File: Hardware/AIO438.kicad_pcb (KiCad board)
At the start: 2 copper layers, 121 x 60 mm, 150 parts, among them J1 5mm screwterminal 01x12, J11 PinHeader 02x03, J12 PinHeader 01x05, J2 JST-PH 01x04, J3 JST-PH 01x03, J4 USB_B_Micro, J5 JST-PH 01x02, J6 JST-PH 01x02, J7 JST-PH 01x10, J8 U.FL, Q2 P-Channel, Q3 N-channel, U1 TAS5825M, U10 CH340C, U11 TPS2113A, U12 ATmega328PB-AU, U2 TAS5825M, U3 TLV1117-33, U4 BTM331, U6 M24256 EEPROM, U7 TPS62177DQC, U8 FE1.1s, Y1 12MHz, Y2 8MHz

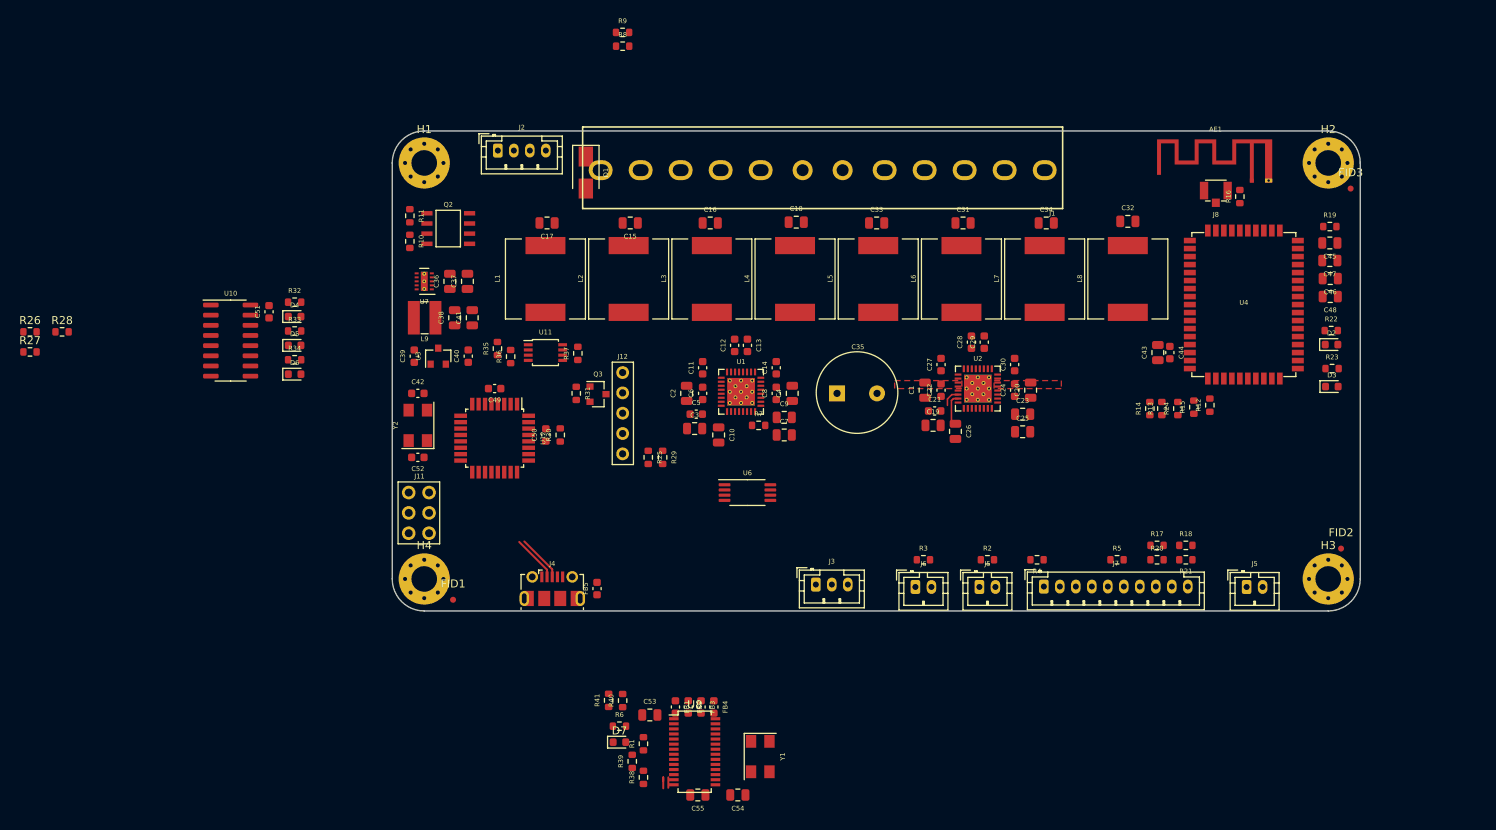
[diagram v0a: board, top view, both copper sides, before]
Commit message: V0.1 check
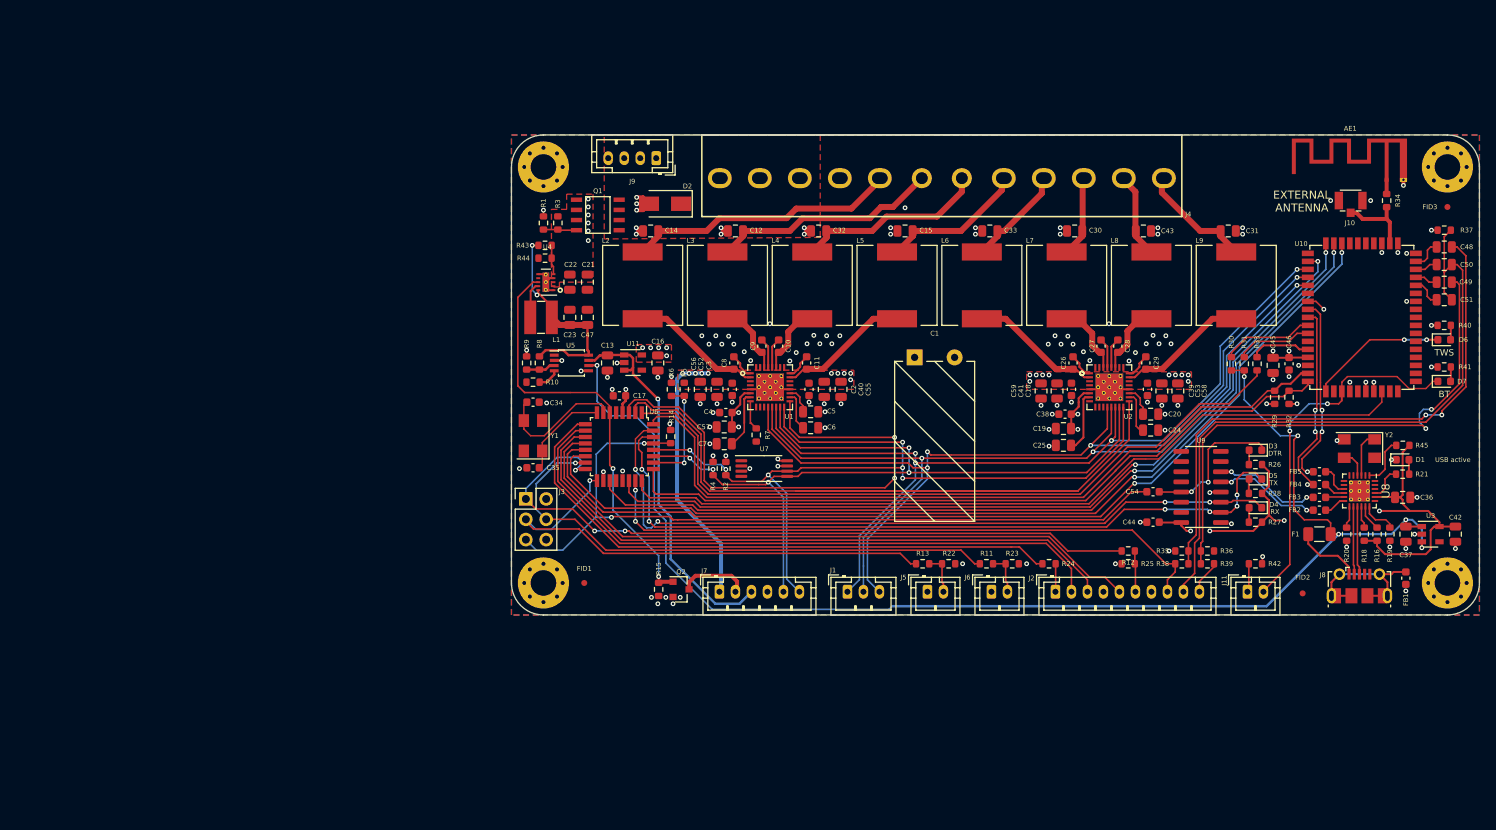
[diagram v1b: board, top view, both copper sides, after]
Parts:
- removed J12: PinHeader 01x05, ZOUDIOfootprints:PinHeader_1x05_P2.54mm_Vertical
- removed the J5 at (194.6, 128.8)
- removed the J5 at (161.2, 128.8)
- removed Q3: N-channel, Package_TO_SOT_SMD:SOT-23
- removed R17: 1k, Resistor_SMD:R_0603_1608Metric
- removed U12: ATmega328PB-AU, Package_QFP:TQFP-32_7x7mm_P0.8mm
- added C56: 22u, Capacitor_SMD:C_0805_2012Metric, F.Cu at (126.3, 104.1)
- added C57: 4.7u, Capacitor_SMD:C_0805_2012Metric, F.Cu at (129.3, 108.8)
- added C58: 22u, Capacitor_SMD:C_0805_2012Metric, F.Cu at (186.0, 104.3)
- added C59: 22u, Capacitor_SMD:C_0805_2012Metric, F.Cu at (168.9, 104.3)
- added F1: 500mA, Fuse:Fuse_1206_3216Metric, F.Cu at (203.7, 122.2)
- added J10: U.FL, ZOUDIOfootprints:Hirose_U.FL-R-SMT-1, F.Cu at (207.6, 80.5)
- added J5: JST-PH 01x02, Connector_JST:JST_PH_B2B-PH-K_1x02_P2.00mm_Vertical, F.Cu at (154.7, 129.4)
- added J9: JST-PH 01x04, Connector_JST:JST_PH_B4B-PH-K_1x04_P2.00mm_Vertical, F.Cu at (120.8, 75.2)
- added LOGO1: ZOUDIO, ZOUDIOfootprints:ZOUDIO25mm, B.Cu at (201.6, 76.5)
- added Q1: P-Channel, ZOUDIOfootprints:SOIC8_mosfet, F.Cu at (113.5, 82.3)
- added R42: 1k, Resistor_SMD:R_0603_1608Metric, F.Cu at (195.7, 125.9)
- added R43: 525k, Resistor_SMD:R_0603_1608Metric, F.Cu at (106.9, 86.1)
- added R44: 100k, Resistor_SMD:R_0603_1608Metric, F.Cu at (106.9, 87.7)
- added R45: 10k, Resistor_SMD:R_0603_1608Metric, F.Cu at (214.1, 111.1)
- added U5: TPS2113A, Package_SO:TSSOP-8_3x3mm_P0.65mm, F.Cu at (110.2, 100.8)
- added U9: CH340B, Package_SO:SOIC-16_3.9x9.9mm_P1.27mm, F.Cu at (188.9, 116.3)
- C1: value 1u -> 820u; footprint Capacitor_SMD:C_0805_2012Metric -> ZOUDIOfootprints:Cap_Rad_D10_P5_horizontal
- C10, C26, C9: value 1u -> 470n; footprint Capacitor_SMD:C_0805_2012Metric -> Capacitor_SMD:C_0603_1608Metric
- C12, C14, C30: value 470n -> 680n; footprint Capacitor_SMD:C_0603_1608Metric -> Capacitor_SMD:C_0805_2012Metric
- C13: value 470n -> 1u; footprint Capacitor_SMD:C_0603_1608Metric -> Capacitor_SMD:C_0805_2012Metric
- C15, C31, C32, C33: value 470n -> 680n
- C16: value 470n -> 1u
- C17, C18: value 470n -> 100n; footprint Capacitor_SMD:C_0805_2012Metric -> Capacitor_SMD:C_0603_1608Metric
- C2, C3, C4, C46: value 1u -> 100n; footprint Capacitor_SMD:C_0805_2012Metric -> Capacitor_SMD:C_0603_1608Metric
- C21, C22, C24, C49, C5, C50, C51, C6: value 100n -> 1u; footprint Capacitor_SMD:C_0603_1608Metric -> Capacitor_SMD:C_0805_2012Metric
- C23, C36, C47: value 1u -> 10u
- C34: value 470n -> 18p; footprint Capacitor_SMD:C_0805_2012Metric -> Capacitor_SMD:C_0603_1608Metric
- C35: value 910u -> 18p; footprint ZOUDIOfootprints:Cap_Rad_D10_P5 -> Capacitor_SMD:C_0603_1608Metric
- C38, C54: value 10u -> 100n; footprint Capacitor_SMD:C_0805_2012Metric -> Capacitor_SMD:C_0603_1608Metric
- C40: value 100n -> 22u; footprint Capacitor_SMD:C_0603_1608Metric -> Capacitor_SMD:C_0805_2012Metric
- C41, C53, C55: value 10u -> 22u
- C42: value 18p -> 1u; footprint Capacitor_SMD:C_0603_1608Metric -> Capacitor_SMD:C_0805_2012Metric
- C43: value 1u -> 680n
- C52: value 18p -> 22u; footprint Capacitor_SMD:C_0603_1608Metric -> Capacitor_SMD:C_0805_2012Metric
- C8: value 100n -> 470n
- D1: value 26V -> Blue; footprint Diode_SMD:D_SMA -> LED_SMD:LED_0603_1608Metric
- D2: value Blue -> 26V; footprint LED_SMD:LED_0603_1608Metric -> Diode_SMD:D_SMA
- J1: value 5mm screwterminal 01x12 -> JST-PH 01x03; footprint ZOUDIOfootprints:Multicomp_12P_5mm -> Connector_JST:JST_PH_B3B-PH-K_1x03_P2.00mm_Vertical
- J11: value PinHeader 02x03 -> JST-PH 01x02; footprint ZOUDIOfootprints:PinSocket_2x03_P2.54mm_Vertical -> Connector_JST:JST_PH_B2B-PH-K_1x02_P2.00mm_Vertical
- J2: value JST-PH 01x04 -> JST-PH 01x10; footprint Connector_JST:JST_PH_B4B-PH-K_1x04_P2.00mm_Vertical -> Connector_JST:JST_PH_B10B-PH-K_1x10_P2.00mm_Vertical
- J3: value JST-PH 01x03 -> PinHeader 02x03; footprint Connector_JST:JST_PH_B3B-PH-K_1x03_P2.00mm_Vertical -> Connector_PinHeader_2.54mm:PinHeader_2x03_P2.54mm_Vertical
- J4: value USB_B_Micro -> 5mm screwterminal 01x12; footprint Connector_USB:USB_Micro-B_Molex-105017-0001 -> ZOUDIOfootprints:Multicomp_12P_5mm
- J7: value JST-PH 01x10 -> PinHeader 01x06; footprint Connector_JST:JST_PH_B10B-PH-K_1x10_P2.00mm_Vertical -> Connector_JST:JST_PH_B6B-PH-K_1x06_P2.00mm_Vertical
- J8: value U.FL -> USB_B_Micro; footprint ZOUDIOfootprints:Hirose_U.FL-R-SMT-1 -> Connector_USB:USB_Micro-B_Molex-105017-0001
- L1: footprint ZOUDIOfootprints:Murata_1274AS-H-100M -> ZOUDIOfootprints:SRN4012TA
- L9: footprint ZOUDIOfootprints:SRN4012TA -> ZOUDIOfootprints:Murata_1274AS-H-100M
- Q2: value P-Channel -> N-channel; footprint ZOUDIOfootprints:SOIC8_mosfet -> Package_TO_SOT_SMD:SOT-23
- R1: value 2k7 -> 1M
- R10: value 1M -> 1K
- R11, R2, R41: value 100k -> 10k
- R13, R14, R19: value 0R -> 10k
- R16: value 0R -> 100k
- R18, R6: value 1k -> 100k
- R20: value 1k -> 2k7
- R22, R23, R25: value 10k -> 100k
- R24, R39: value 10k -> 1k
- R30, R31, R34: value 10k -> 0R
- R35, R36, R38: value 100k -> 1k
- R37: value 500R -> 0R
- R4: value 100R -> 10k
- R40: value 47k -> 10k
- R5: value 100k -> 1M
- R8: value 1M -> 10k
- U10: value CH340C -> BTM331; footprint Package_SO:SOIC-16_3.9x9.9mm_P1.27mm -> ZOUDIOfootprints:BTM331
- U11: value TPS2113A -> LP5907MFX-3.3; footprint Package_SO:TSSOP-8_3x3mm_P0.65mm -> Package_TO_SOT_SMD:SOT-23-5
- U3: value TLV1117-33 -> LP5907MFX-3.3; footprint Package_TO_SOT_SMD:SOT-23 -> Package_TO_SOT_SMD:SOT-23-5
- U4: value BTM331 -> TPS62175DQC; footprint ZOUDIOfootprints:BTM331 -> Package_SON:WSON-10-1EP_2x3mm_P0.5mm_EP0.84x2.4mm_ThermalVias
- U6: value M24256 EEPROM -> ATmega328PB-AU; footprint Package_SO:TSSOP-8_4.4x3mm_P0.65mm -> Package_QFP:TQFP-32_7x7mm_P0.8mm
- U7: value TPS62177DQC -> M24256 EEPROM; footprint Package_SON:WSON-10-1EP_2x3mm_P0.5mm_EP0.84x2.4mm_ThermalVias -> Package_SO:TSSOP-8_4.4x3mm_P0.65mm
- U8: value FE1.1s -> FE1.1s-BQFN24B; footprint Package_SO:SSOP-28_3.9x9.9mm_P0.635mm -> Package_DFN_QFN:QFN-24-1EP_4x4mm_P0.5mm_EP2.6x2.6mm_ThermalVias
- Y1: value 12MHz -> 8MHz
- Y2: value 8MHz -> 12MHz
- moved R27 154.7 mm to (195.7, 120.7), turned to 180 degrees
- moved R26 154.1 mm to (195.7, 113.5), turned to 180 degrees
- moved R28 150.5 mm to (195.7, 117.1), turned to 180 degrees
- moved C51 146.9 mm to (219.3, 92.9), turned to 180 degrees
- moved D6 143.8 mm to (219.3, 97.9)
- moved R34 137.9 mm to (212.1, 80.5), turned to 90 degrees
- moved U10 135.3 mm to (202.5, 87.1)
- moved C42 130.9 mm to (220.7, 122.2), turned to 270 degrees
- moved U3 126.0 mm to (217.6, 122.2), turned to 0 degrees
- moved R32 124.9 mm to (199.9, 105.1), turned to 90 degrees
- moved D4 122.5 mm to (195.7, 118.9), turned to 180 degrees
- moved C36 122.1 mm to (214.1, 117.6), turned to 180 degrees
- moved C37 121.5 mm to (214.5, 122.2), turned to 270 degrees
- moved D5 121.3 mm to (195.7, 115.3), turned to 180 degrees
- moved R33 120.4 mm to (195.9, 100.9), turned to 270 degrees
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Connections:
- C1 pad 1: GND -> VDD
- C1 pad 2: VDD -> GND
- C10 pad 2: GND -> Net-(C10-Pad2)
- C12 pad 1: Net-(C12-Pad1) -> GND
- C12 pad 2: Net-(C12-Pad2) -> /Amplifiers/A-
- C13 pad 1: Net-(C13-Pad1) -> +5V
- C13 pad 2: Net-(C13-Pad2) -> GND
- C14 pad 1: Net-(C14-Pad1) -> GND
- C14 pad 2: Net-(C14-Pad2) -> /Amplifiers/A+
- C15 pad 2: /Amplifiers/A- -> /Amplifiers/B+
- C16 pad 1: GND -> +3V3
- C16 pad 2: /Amplifiers/B+ -> GND
- C17 pad 1: GND -> +3V3
- C17 pad 2: /Amplifiers/A+ -> GND
- C18 pad 2: /Amplifiers/B- -> VDD
- C20 pad 1: GND -> Net-(C20-Pad1)
- C20 pad 2: VDD -> GND
- C21 pad 2: +3V3 -> VDD
- C23 pad 1: Net-(C23-Pad1) -> /Power/5V_buck
- C24 pad 1: GND -> Net-(C24-Pad1)
- C24 pad 2: VDD -> GND
- C26 pad 2: GND -> Net-(C26-Pad2)
- C3 pad 2: +3V3 -> VDD
- C30 pad 1: Net-(C30-Pad1) -> GND
- C30 pad 2: Net-(C30-Pad2) -> /Amplifiers/C-
- C31 pad 2: /Amplifiers/C- -> /Amplifiers/D+
- C32 pad 2: /Amplifiers/D+ -> /Amplifiers/B-
- C34 pad 1: GND -> /Microcontroller/XTAL1
- C34 pad 2: /Amplifiers/D- -> GND
- C35 pad 1: VDD -> /Microcontroller/XTAL2
- C36 pad 2: VDD -> /USB/3V3
- C37 pad 1: GND -> 5V_usb
- C37 pad 2: VDD -> GND
- C38 pad 1: /Power/3V3_buck -> GND
- C38 pad 2: GND -> +3V3
- C39 pad 1: +5V -> GND
- C39 pad 2: GND -> VDD
- C4 pad 2: VDD -> +3V3
- C40 pad 2: /Power/3V3_ldo -> VDD
- C41 pad 1: /Power/3V3_buck -> GND
- C41 pad 2: GND -> VDD
- C42 pad 1: /Microcontroller/XTAL1 -> /USB/3V3
- C43 pad 1: +3V3 -> GND
- C43 pad 2: GND -> /Amplifiers/D-
- C44 pad 2: +3V3 -> /USB/3V3
- C45 pad 1: Net-(C45-Pad1) -> +3V3
- C45 pad 2: Net-(C45-Pad2) -> GND
- C46 pad 1: Net-(C46-Pad1) -> GND
- C46 pad 2: Net-(C46-Pad2) -> +3V3
- C47 pad 1: /User controls/AUX_GND -> /Power/5V_buck
- C47 pad 2: Net-(C47-Pad2) -> GND
- C48 pad 1: /User controls/AUX_GND -> Net-(C48-Pad1)
- C49 pad 1: +3V3 -> Net-(C49-Pad1)
- C49 pad 2: GND -> Net-(C49-Pad2)
- C5 pad 1: GND -> Net-(C5-Pad1)
- C5 pad 2: +3V3 -> GND
- C50 pad 1: /Microcontroller/RESET -> /User controls/AUX_GND
- C50 pad 2: /Microcontroller/DTR -> Net-(C50-Pad2)
- C51 pad 1: GND -> /User controls/AUX_GND
- C51 pad 2: +3V3 -> Net-(C51-Pad2)
- C52 pad 1: /Microcontroller/XTAL2 -> GND
- C52 pad 2: GND -> VDD
- C53 pad 2: /USB/3V3 -> VDD
- C54 pad 1: GND -> /Microcontroller/RESET
- C54 pad 2: /USB/1V8 -> /Microcontroller/DTR
- C55 pad 2: +5V -> VDD
- C6 pad 1: GND -> Net-(C6-Pad1)
- C6 pad 2: VDD -> GND
- C8 pad 1: GND -> Net-(C8-Pad1)
- C8 pad 2: VDD -> Net-(C8-Pad2)
- C9 pad 2: GND -> Net-(C9-Pad2)
- D1 pad 1: Vin -> GND
- D1 pad 2: GND -> Net-(D1-Pad2)
- D2 pad 1: /Bluetooth/LED2 -> Vin
- D2 pad 2: Net-(D2-Pad2) -> GND
- D3 pad 1: /Bluetooth/LED5 -> /Microcontroller/DTR
- D4 pad 1: /Microcontroller/DTR -> /USB to UART/UART_RX
- D5 pad 1: /USB to UART/UART_RX -> /Microcontroller/UART_RX
- D6 pad 1: /Microcontroller/UART_RX -> /Bluetooth/LED2
- D7 pad 1: Net-(D7-Pad1) -> /Bluetooth/LED5
- D7 pad 2: /USB/DRV -> Net-(D7-Pad2)
- FB1 pad 1: /USB/DP1 -> GND
- FB2 pad 1: /USB/DM1 -> /USB/D1+
- FB3 pad 1: /USB/DP2 -> /USB/D1-
- FB4 pad 1: /USB/DM2 -> /USB/D2+
- FB5 pad 1: GND -> /USB/D2-
- J1 pad 1: /Amplifiers/D+ -> /Amplifiers/I2S_SDIN
- J1 pad 2: /Amplifiers/D- -> /Amplifiers/I2S_SCLK
- J1 pad 3: /Amplifiers/C- -> /Amplifiers/I2S_LRCLK
- J11 pad 1: +3V3 -> Net-(J11-Pad1)
- J11 pad 2: /Microcontroller/SPI_MISO0 -> /Bluetooth/LED5
- J2 pad 1: GND -> Net-(J2-Pad1)
- J2 pad 2: GND -> /User controls/LED_RED
- J2 pad 3: Vin -> /Microcontroller/PD7
- J2 pad 4: Vin -> GND
- J3 pad 1: /Amplifiers/I2S_SDIN -> /Microcontroller/SPI_MISO0
- J3 pad 2: /Amplifiers/I2S_SCLK -> +3V3
- J3 pad 3: /Amplifiers/I2S_LRCLK -> /Microcontroller/SPI_CLK0
- J4 pad 1: Net-(F1-Pad2) -> /Amplifiers/D+
- J4 pad 2: Net-(J4-Pad2) -> /Amplifiers/D-
- J4 pad 3: Net-(J4-Pad3) -> /Amplifiers/C-
- J4 pad 4: Net-(J4-Pad4) -> /Amplifiers/C+
- J4 pad 5: GND -> /Amplifiers/B+
- J4 pad 6: Net-(FB5-Pad2) -> /Amplifiers/B-
- J7 pad 1: Net-(J7-Pad1) -> VDD
- J7 pad 2: /User controls/LED_RED -> Net-(J7-Pad2)
- J7 pad 3: /Microcontroller/PC3 -> +5V
- J7 pad 4: GND -> +3V3
- J7 pad 5: /Microcontroller/PD4 -> /Amplifiers/I2C_SDA
- J7 pad 6: /Microcontroller/PB1 -> /Amplifiers/I2C_SCL
- J8 pad 1: GND -> Net-(F1-Pad2)
- J8 pad 3: GND -> Net-(J8-Pad3)
- L1 pad 1: Net-(C11-Pad1) -> Net-(L1-Pad1)
- L1 pad 2: /Amplifiers/A+ -> /Power/5V_buck
- L2 pad 1: Net-(C12-Pad1) -> Net-(C8-Pad1)
- L2 pad 2: /Amplifiers/A- -> /Amplifiers/A+
- L3 pad 1: Net-(C13-Pad1) -> Net-(C9-Pad1)
- L3 pad 2: /Amplifiers/B- -> /Amplifiers/A-
- L4 pad 1: Net-(C14-Pad1) -> Net-(C10-Pad1)
- L4 pad 2: /Amplifiers/B+ -> /Amplifiers/B-
- L5 pad 1: Net-(C27-Pad1) -> Net-(C11-Pad1)
- L5 pad 2: /Amplifiers/C+ -> /Amplifiers/B+
- L6 pad 1: Net-(C28-Pad1) -> Net-(C26-Pad1)
- L6 pad 2: /Amplifiers/C- -> /Amplifiers/C+
- L7 pad 1: Net-(C29-Pad1) -> Net-(C27-Pad1)
- L7 pad 2: /Amplifiers/D- -> /Amplifiers/C-
- L8 pad 1: Net-(C30-Pad1) -> Net-(C28-Pad1)
- L8 pad 2: /Amplifiers/D+ -> /Amplifiers/D-
- L9 pad 1: Net-(L9-Pad1) -> Net-(C29-Pad1)
- L9 pad 2: /Power/3V3_buck -> /Amplifiers/D+
- Q2 pad 1: Net-(Q2-Pad1) -> /Power/Buck_sleep
- Q2 pad 2: VDD -> GND
- Q2 pad 3: Vin -> Net-(J7-Pad2)
- R1 pad 1: GND -> Net-(Q1-Pad1)
- R1 pad 2: Net-(R1-Pad2) -> GND
- R10 pad 1: Net-(Q2-Pad1) -> Net-(R10-Pad1)
- R11 pad 1: VDD -> /User controls/EQ_SW
- R11 pad 2: Net-(Q2-Pad1) -> /Microcontroller/SPI_MOSI0
- R12 pad 1: +3V3 -> /Microcontroller/PB4
- R12 pad 2: /Bluetooth/LED0 -> /Microcontroller/SPI_MISO0
- R13 pad 1: Net-(R13-Pad1) -> /Microcontroller/PB5
- R13 pad 2: +5V -> /Microcontroller/SPI_CLK0
- R14 pad 1: Net-(R14-Pad1) -> /Microcontroller/RESET
- R14 pad 2: +5V -> +3V3
- R15 pad 1: +3V3 -> /Power/Buck_sleep
- R15 pad 2: /Bluetooth/LED1 -> GND
- R16 pad 1: Net-(J8-Pad2) -> /USB/3V3
- R16 pad 2: Net-(AE1-Pad1) -> Net-(R16-Pad2)
- R18 pad 1: GND -> /USB/3V3
- R18 pad 2: Net-(C46-Pad1) -> Net-(R18-Pad2)
- R19 pad 2: /User controls/AUX_GND -> Net-(R19-Pad2)
- R2 pad 1: /Microcontroller/PB0 -> +3V3
- R2 pad 2: GND -> /Amplifiers/I2C_SCL
- R20 pad 1: /User controls/AUX_R -> GND
- R20 pad 2: Net-(C45-Pad1) -> Net-(R20-Pad2)
- R21 pad 1: /User controls/AUX_L -> /USB/DRV
- R21 pad 2: Net-(C46-Pad1) -> Net-(D1-Pad2)
- R22 pad 1: +3V3 -> /Microcontroller/PB5
- R22 pad 2: Net-(D2-Pad2) -> GND
- R23 pad 1: +3V3 -> /User controls/EQ_SW
- R23 pad 2: Net-(D3-Pad2) -> GND
- R24 pad 1: Net-(R24-Pad1) -> Net-(J2-Pad1)
- R24 pad 2: /Bluetooth/Enable -> /User controls/LED_GREEN
- R25 pad 1: +3V3 -> GND
- R25 pad 2: /Amplifiers/I2C_SCL -> /Microcontroller/PB4
- R26 pad 1: /User controls/LED_GREEN -> /USB/3V3
- R26 pad 2: /Microcontroller/SPI_MOSI0 -> Net-(D3-Pad2)
- R27 pad 1: /User controls/EQ_SW -> /USB/3V3
- R27 pad 2: /Microcontroller/SPI_MISO0 -> Net-(D4-Pad2)
- R28 pad 1: /Microcontroller/PB5 -> /USB/3V3
- R28 pad 2: /Microcontroller/SPI_CLK0 -> Net-(D5-Pad2)
- R29 pad 2: /Amplifiers/I2C_SDA -> /Bluetooth/LED0
- R3 pad 1: /User controls/EQ_SW -> VDD
- R3 pad 2: GND -> Net-(Q1-Pad1)
- R30 pad 1: /Microcontroller/RESET -> Net-(R30-Pad1)
- R30 pad 2: +3V3 -> 5V_usb
- R31 pad 1: /Microcontroller/PE1 -> Net-(R31-Pad1)
- R31 pad 2: GND -> 5V_usb
- R32 pad 2: Net-(D4-Pad2) -> /Bluetooth/LED1
- R33 pad 1: +3V3 -> Net-(R33-Pad1)
- R33 pad 2: Net-(D5-Pad2) -> /Bluetooth/Enable
- R34 pad 1: +3V3 -> Net-(J10-Pad2)
- R34 pad 2: Net-(D6-Pad2) -> Net-(AE1-Pad1)
- R35 pad 1: Net-(R35-Pad1) -> GND
- R35 pad 2: /Power/3V3_ldo -> Net-(C48-Pad1)
- R36 pad 2: Net-(R35-Pad1) -> Net-(C49-Pad1)
- R37 pad 1: Net-(R37-Pad1) -> GND
- R37 pad 2: GND -> /User controls/AUX_GND
- R38 pad 1: +5V -> /User controls/AUX_L
- R38 pad 2: Net-(R38-Pad2) -> Net-(C48-Pad1)
- R39 pad 1: GND -> /User controls/AUX_R
- R39 pad 2: Net-(R39-Pad2) -> Net-(C49-Pad1)
- R4 pad 1: Net-(J7-Pad1) -> +3V3
- R4 pad 2: /User controls/LED_GREEN -> /Amplifiers/I2C_SDA
- R40 pad 1: +5V -> +3V3
- R40 pad 2: Net-(R40-Pad2) -> Net-(D6-Pad2)
- R41 pad 1: Net-(R40-Pad2) -> +3V3
- R41 pad 2: GND -> Net-(D7-Pad2)
- R5 pad 1: GND -> VDD
- R5 pad 2: /Microcontroller/PB1 -> /Microcontroller/PC3
- R6 pad 1: Net-(D7-Pad1) -> /Microcontroller/PC3
- R8 pad 1: VDD -> Net-(R8-Pad1)
- R8 pad 2: /Microcontroller/PD7 -> /Power/5V_buck
- R9 pad 1: /Microcontroller/PD7 -> GND
- R9 pad 2: GND -> Net-(R8-Pad1)
- U1 pad 1: Net-(C11-Pad2) -> Net-(C8-Pad2)
- U1 pad 18: Net-(C9-Pad1) -> Net-(C6-Pad1)
- U1 pad 19: Net-(C7-Pad1) -> Net-(C5-Pad1)
- U1 pad 2: Net-(C11-Pad1) -> Net-(C8-Pad1)
- U1 pad 23: Net-(C14-Pad1) -> Net-(C11-Pad1)
- U1 pad 24: Net-(C14-Pad2) -> Net-(C11-Pad2)
- U1 pad 27: Net-(C13-Pad1) -> Net-(C10-Pad1)
- U1 pad 28: Net-(C13-Pad2) -> Net-(C10-Pad2)
- U1 pad 29: Net-(C12-Pad2) -> Net-(C9-Pad2)
- U1 pad 30: Net-(C12-Pad1) -> Net-(C9-Pad1)
- U1 pad 7: Net-(C10-Pad1) -> Net-(C7-Pad1)
- U10 pad 1: GND -> Net-(U10-Pad1)
- U10 pad 10: Net-(U10-Pad10) -> Net-(R30-Pad1)
- U10 pad 11: Net-(U10-Pad11) -> Net-(R31-Pad1)
- U10 pad 13: /Microcontroller/DTR -> Net-(R33-Pad1)
- U10 pad 14: Net-(U10-Pad14) -> +3V3
- U10 pad 15: Net-(U10-Pad15) -> GND
- U10 pad 16: +3V3 -> /Bluetooth/LED0
- U10 pad 2: /Microcontroller/UART_RX -> /Microcontroller/PE3
- U10 pad 3: /USB to UART/UART_RX -> /Amplifiers/I2S_SDIN
- U10 pad 4: +3V3 -> /Amplifiers/I2S_LRCLK
- U10 pad 5: /USB/DP1 -> /Amplifiers/I2S_SCLK
- U10 pad 6: /USB/DM1 -> Net-(U10-Pad6)
- U10 pad 7: Net-(U10-Pad7) -> +3V3
- U10 pad 8: Net-(U10-Pad8) -> /USB/D2-
- U10 pad 9: Net-(U10-Pad9) -> /USB/D2+
- U11 pad 1: Net-(U11-Pad1) -> +5V
- U11 pad 3: Net-(R35-Pad1) -> +5V
- U11 pad 4: Net-(R37-Pad1) -> Net-(U11-Pad4)
- U11 pad 5: GND -> +3V3
- U2 pad 1: Net-(C27-Pad2) -> Net-(C26-Pad2)
- U2 pad 18: Net-(C25-Pad1) -> Net-(C24-Pad1)
- U2 pad 19: Net-(C23-Pad1) -> Net-(C20-Pad1)
- U2 pad 2: Net-(C27-Pad1) -> Net-(C26-Pad1)
- U2 pad 23: Net-(C30-Pad1) -> Net-(C29-Pad1)
- U2 pad 24: Net-(C30-Pad2) -> Net-(C29-Pad2)
- U2 pad 27: Net-(C29-Pad1) -> Net-(C28-Pad1)
- U2 pad 28: Net-(C29-Pad2) -> Net-(C28-Pad2)
- U2 pad 29: Net-(C28-Pad2) -> Net-(C27-Pad2)
- U2 pad 30: Net-(C28-Pad1) -> Net-(C27-Pad1)
- U2 pad 7: Net-(C26-Pad1) -> Net-(C25-Pad1)
- U3 pad 1: GND -> 5V_usb
- U3 pad 2: /Power/3V3_ldo -> GND
- U3 pad 3: +5V -> 5V_usb
- U4 pad 1: Net-(U4-Pad1) -> GND
- U4 pad 10: Net-(R13-Pad1) -> /Power/5V_buck
- U4 pad 11: Net-(R14-Pad1) -> GND
- U4 pad 2: /Microcontroller/PC1 -> VDD
- U4 pad 3: /Amplifiers/I2S_SDIN -> VDD
- U4 pad 4: /Amplifiers/I2S_LRCLK -> GND
- U4 pad 5: /Amplifiers/I2S_SCLK -> Net-(R43-Pad2)
- U4 pad 6: Net-(U4-Pad6) -> GND
- U4 pad 7: +3V3 -> Net-(U4-Pad7)
- U4 pad 8: /USB/DM2 -> /Power/Buck_sleep
- U4 pad 9: /USB/DP2 -> Net-(L1-Pad1)
- U6 pad 1: GND -> /Bluetooth/Enable
- U6 pad 2: GND -> /Amplifiers/AMP2_PDN
- U6 pad 3: GND -> /Amplifiers/AMP1_PDN
- U6 pad 4: GND -> +3V3
- U6 pad 5: /Amplifiers/I2C_SDA -> GND
- U6 pad 6: /Amplifiers/I2C_SCL -> /Power/Buck_sleep
- U6 pad 7: GND -> /Microcontroller/XTAL1
- U6 pad 8: +3V3 -> /Microcontroller/XTAL2
- U7 pad 2: VDD -> GND
- U7 pad 3: VDD -> GND
- U7 pad 5: GND -> /Amplifiers/I2C_SDA
- U7 pad 6: GND -> /Amplifiers/I2C_SCL
- U7 pad 7: Net-(U7-Pad7) -> GND
- U7 pad 8: /Power/Buck_sleep -> +3V3
- U8 pad 1: GND -> Net-(R45-Pad2)
- U8 pad 10: Net-(FB2-Pad2) -> Net-(FB4-Pad2)
- U8 pad 11: Net-(FB1-Pad2) -> Net-(FB3-Pad2)
- U8 pad 12: /USB/1V8 -> Net-(FB2-Pad2)
- U8 pad 13: /USB/3V3 -> Net-(R20-Pad2)
- U8 pad 14: Net-(R1-Pad2) -> Net-(J8-Pad2)
- U8 pad 15: Net-(J4-Pad2) -> Net-(J8-Pad3)
- U8 pad 16: Net-(J4-Pad3) -> Net-(R18-Pad2)
- U8 pad 17: Net-(R38-Pad2) -> Net-(R16-Pad2)
- U8 pad 18: Net-(R40-Pad2) -> Net-(R19-Pad2)
- U8 pad 19: Net-(R39-Pad2) -> Net-(U8-Pad19)
- U8 pad 2: Net-(U8-Pad2) -> /USB/I2C_SDA
- U8 pad 20: +5V -> /USB/3V3
- U8 pad 21: /USB/3V3 -> /USB/DRV
- U8 pad 22: /USB/DRV -> /USB/I2C_SCL
- U8 pad 23: /USB/I2C_SCL -> /USB/LED2
- U8 pad 24: /USB/LED2 -> Net-(U8-Pad24)
- U8 pad 25: Net-(U8-Pad25) -> GND
- U8 pad 8: Net-(FB4-Pad2) -> Net-(U8-Pad8)
- U8 pad 9: Net-(FB3-Pad2) -> Net-(FB5-Pad2)
- Y1 pad 1: Net-(U8-Pad2) -> /Microcontroller/XTAL2
- Y1 pad 3: GND -> /Microcontroller/XTAL1
- Y1 pad 4: Net-(U8-Pad3) -> GND
- Y2 pad 1: /Microcontroller/XTAL2 -> Net-(U8-Pad3)
- Y2 pad 3: GND -> Net-(U8-Pad4)
- Y2 pad 4: /Microcontroller/XTAL1 -> GND
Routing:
- net 5V_usb: track 0.00 -> 170.0 mm, vias 0 -> 6
- net /Microcontroller/PB1: track 0.00 -> 121.9 mm, vias 0 -> 2
- net /Microcontroller/PB2: track 0.00 -> 119.1 mm, vias 0 -> 2
- net /Amplifiers/AMP2_PDN: track 0.00 -> 113.5 mm
- net /Amplifiers/I2S_LRCLK: track 0.00 -> 111.0 mm, vias 0 -> 4
- net /Microcontroller/PE2: track 0.00 -> 109.4 mm, vias 0 -> 2
- net /Amplifiers/I2S_SCLK: track 0.00 -> 108.7 mm, vias 0 -> 3
- net /Amplifiers/I2S_SDIN: track 0.00 -> 108.4 mm, vias 0 -> 4
- net /Amplifiers/I2C_SCL: track 0.00 -> 106.7 mm, vias 0 -> 6
- net /Microcontroller/PE3: track 0.00 -> 105.2 mm, vias 0 -> 2
- net /Amplifiers/I2C_SDA: track 0.00 -> 103.9 mm, vias 0 -> 5
- net /Microcontroller/PC1: track 0.00 -> 101.0 mm
- net /Microcontroller/RESET: track 0.00 -> 100.0 mm, vias 0 -> 2
- net /Bluetooth/LED0: track 0.00 -> 96.6 mm
- net /Microcontroller/UART_RX: track 0.00 -> 95.0 mm, vias 0 -> 6
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- added copper zone on F.Cu, net +3V3
- added copper zone on In2.PWR, net +3V3
- added copper zone on B.Cu, net GND
- added copper zone on F.Cu, net GND
- added copper zone on In1.GND, net GND
- added copper zone on In2.PWR, net VDD
- added copper zone on F.Cu, net Vin
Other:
- copper layers 2 -> 4
- net class Default: clearance 0.2 -> 0.1778; trace_width 0.25 -> 0.1778; via_dia 0.8 -> 0.6; via_drill 0.4 -> 0.3
- rule trace_clearance: 0.2 -> 0.1778
- rule trace_min: 0.2 -> 0.1778
- rule via_min_size: 0.4 -> 0.3
- board text added: "+"
- board text added: "-"
- board text added: "A"
- board text added: "AUX"
- board text added: "B"
- board text added: "BT"
- board text added: "BT LED"
- board text added: "C"
- board text added: "CHG"
- board text added: "D"
- board text added: "DTR"
- board text added: "EQ"
- board text added: "EXTERNAL ANTENNA"
- board text added: "Expansion"
- board text added: "I2S"
- board text added: "LED"
- board text added: "PSU"
- board text added: "ROT"
- board text added: "RX"
- board text added: "TWS"
- board text added: "TX"
- board text added: "USB active"
- board text added: "ZOUDIO AIO438 www.ZOUDIO.com The Netherlands"
